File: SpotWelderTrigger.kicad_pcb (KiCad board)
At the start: 2 copper layers, 91.4 x 77.5 mm, 36 parts, among them J1 230VAC, J2 ToTransformer, J3 Conn_01x05_Male, J4 Conn_01x02_Male, T1 TYN616, T2 TYN616, U1 EL817, U2 MOC3021M, U3 LM7805_TO220

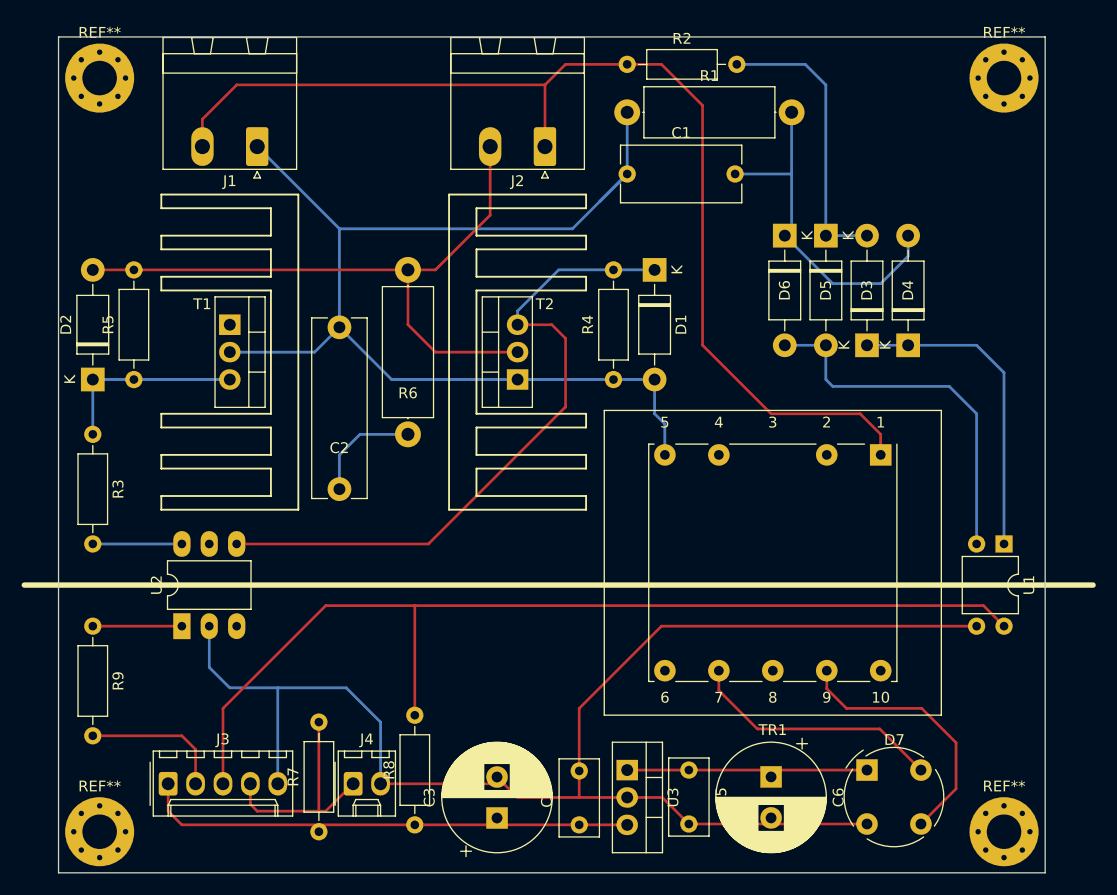
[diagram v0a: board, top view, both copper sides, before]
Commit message: Full layout
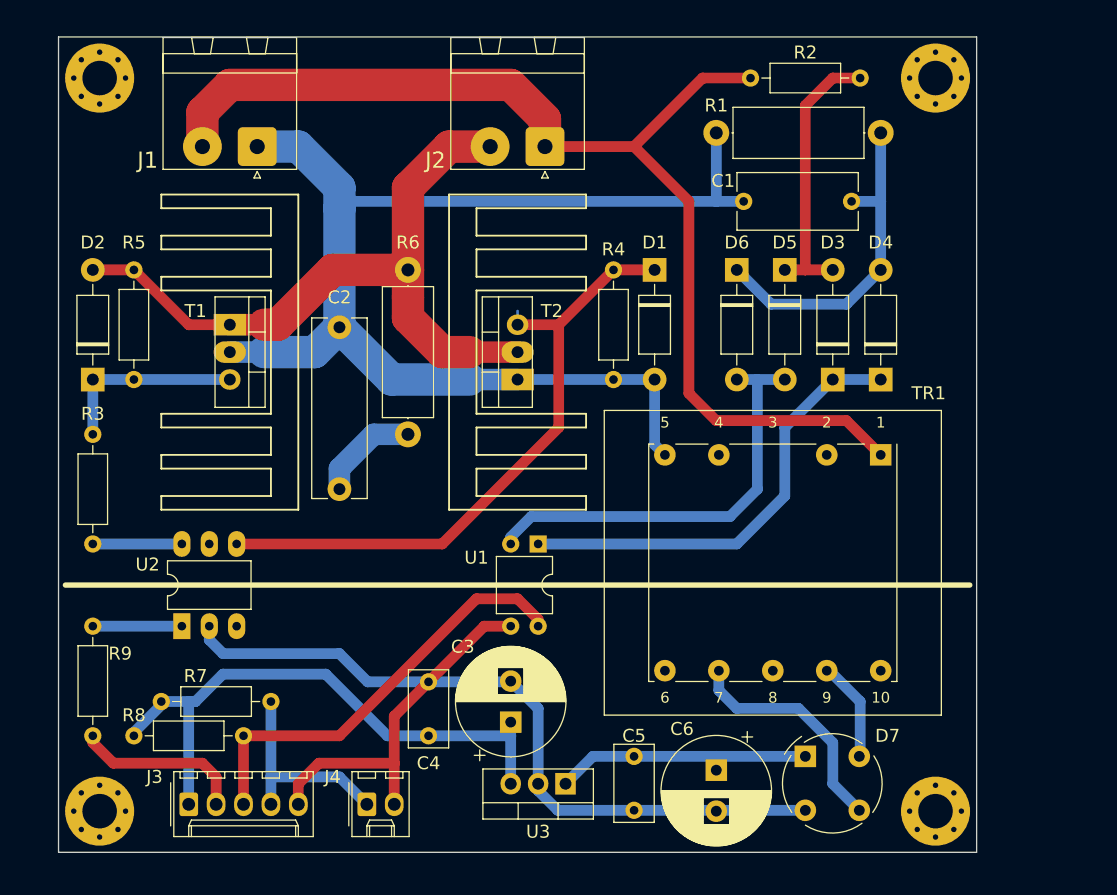
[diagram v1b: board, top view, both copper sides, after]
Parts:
- removed the REF** at (179.7, 48.3)
- removed the REF** at (95.9, 118.1)
- added REF**: MountingHole_3.2mm_M3_Pad_Via, MountingHole:MountingHole_3.2mm_M3_Pad_Via, F.Cu at (173.4, 48.3)
- added REF**: MountingHole_3.2mm_M3_Pad_Via, MountingHole:MountingHole_3.2mm_M3_Pad_Via, F.Cu at (95.9, 116.2)
- moved U1 43.2 mm to (136.5, 91.4)
- moved R8 27.3 mm to (99.1, 109.2), turned to 0 degrees
- moved R7 18.9 mm to (101.6, 106.0), turned to 0 degrees
- moved C4 16.2 mm to (126.4, 109.2)
- moved R2 11.5 mm to (156.2, 48.3)
- moved C1 11.1 mm to (155.6, 59.7)
- moved C3 8.98 mm to (134.0, 108.0)
- moved R1 8.47 mm to (153.0, 53.3)
- moved REF** 6.63 mm to (173.4, 116.2)
- moved U3 5.85 mm to (139.1, 113.7), turned to 180 degrees
- moved D7 5.85 mm to (161.3, 111.1)
- moved D6 5.46 mm to (154.9, 66.0)
- moved C5 5.24 mm to (145.4, 111.1)
- moved C6 5.12 mm to (153.0, 112.4)
- moved D5 4.96 mm to (159.4, 66.0)
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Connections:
- TR1 pad 7: Net-(D7-Pad4) -> Net-(D7-Pad3)
- TR1 pad 9: Net-(D7-Pad3) -> Net-(D7-Pad4)
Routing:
- net Net-(J3-Pad3): track 94.3 -> 40.3 mm
- net GND: track 133.2 -> 102.4 mm
- net Net-(D7-Pad4): track 23.6 -> 9.39 mm
- net Net-(D3-Pad1): track 29.6 -> 41.8 mm
- net Net-(C1-Pad1): track 107.7 -> 117.1 mm
- net VCC: track 46.9 -> 55.3 mm
- net Net-(D5-Pad2): track 34.3 -> 39.9 mm
- net Net-(J1-Pad2): track 102.4 -> 106.6 mm
- net Net-(D2-Pad2): track 61.6 -> 64.9 mm
- net Net-(D7-Pad3): track 24.6 -> 21.7 mm
- net Net-(J3-Pad2): track 13.2 -> 15.9 mm
- net Net-(D1-Pad1): track 62.6 -> 59.9 mm
- net Net-(C1-Pad2): track 33.2 -> 31.4 mm
- net Net-(C5-Pad1): track 22.9 -> 24.6 mm
- net Net-(J3-Pad4): track 21.0 -> 19.5 mm
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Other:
- board size 91.4 x 77.5 mm -> 85.1 x 75.6 mm
